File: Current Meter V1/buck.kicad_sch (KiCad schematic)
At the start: 13 parts, among them SW1 SW_DIP_x01, U2 TPS5430DDAR

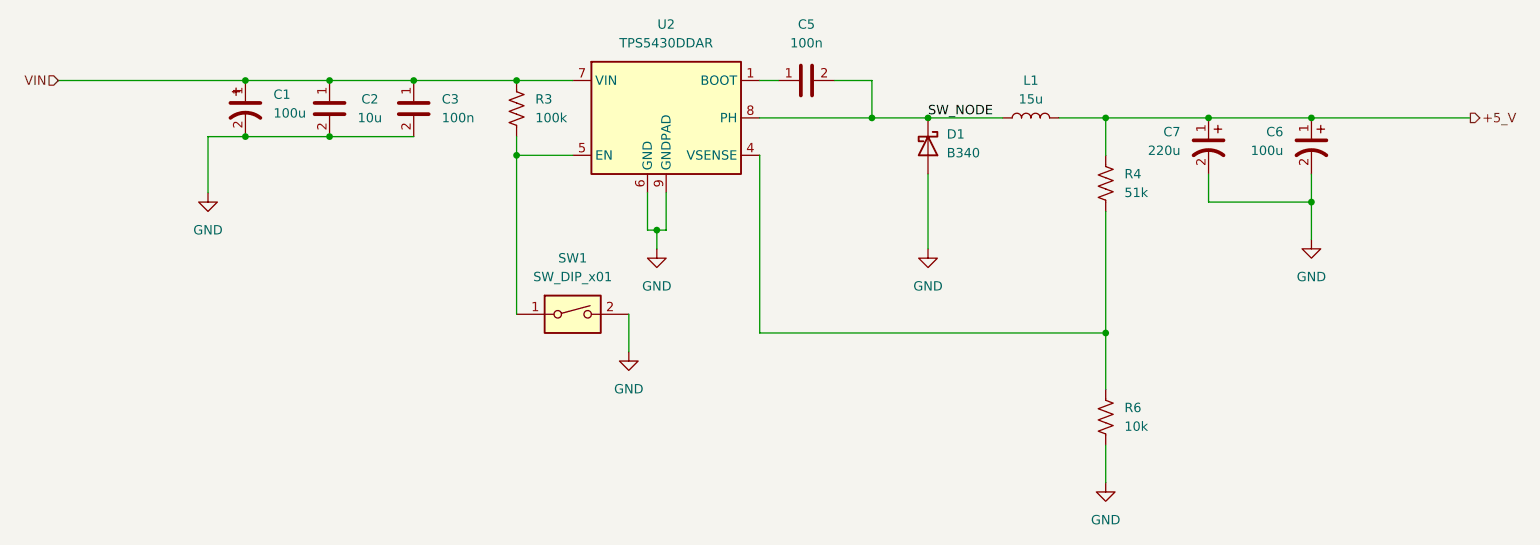
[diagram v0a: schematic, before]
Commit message: buck
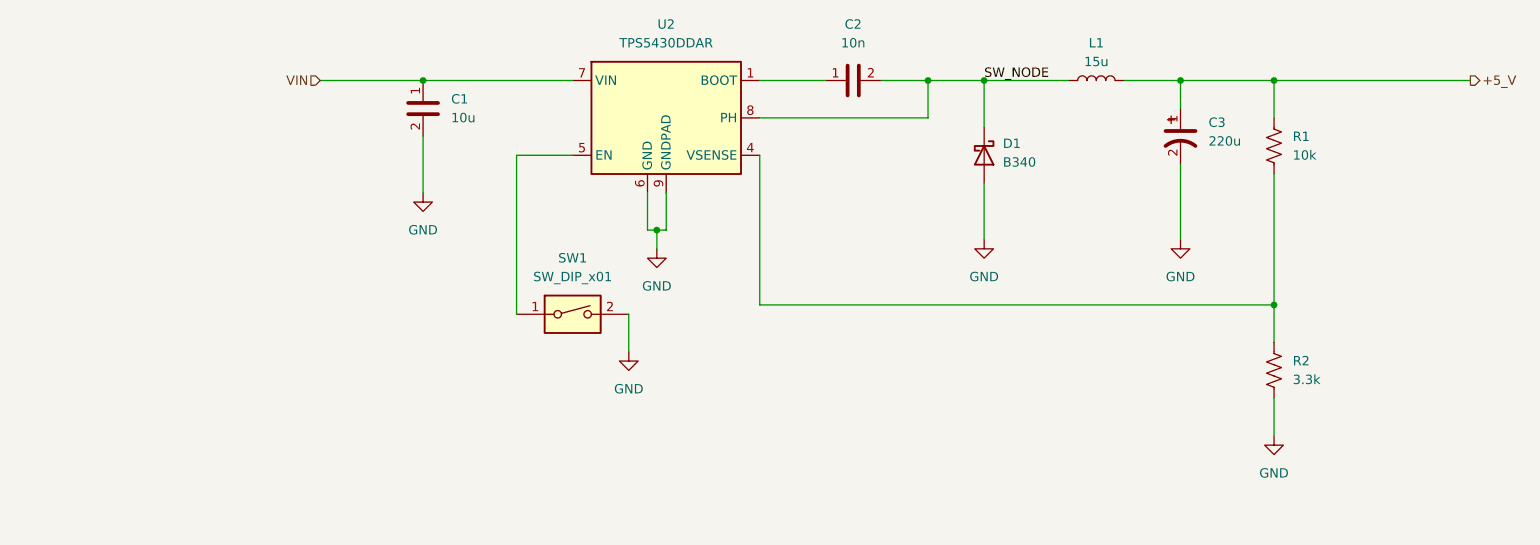
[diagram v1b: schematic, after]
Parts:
- removed C1, C6: 100u, Capacitor_THT:CP_Radial_D8.0mm_P3.50mm, symbol bfr_capacitors:50ZLH100MEFC8X11.5
- removed C2: 10u, Capacitor_SMD:C_0603_1608Metric, symbol bfr_capacitors:CL05A106MQ5NUNC
- removed C3, C5: 100n, Capacitor_SMD:C_0402_1005Metric_Pad0.74x0.62mm_HandSolder, symbol bfr_capacitors:CL05B104KB54PNC
- removed C7: 220u, Capacitor_THT:CP_Radial_D8.0mm_P3.50mm, symbol bfr_capacitors:35ZLH220MEFC8X11.5
- removed R3: 100k, Resistor_SMD:R_0402_1005Metric_Pad0.72x0.64mm_HandSolder, symbol bfr_resistors:RMCF0402FT100K
- removed R4: 51k, Resistor_SMD:R_0402_1005Metric_Pad0.72x0.64mm_HandSolder, symbol bfr_resistors:RMCF0402FT51K0
- removed R6: 10k, Resistor_SMD:R_0402_1005Metric_Pad0.72x0.64mm_HandSolder, symbol bfr_resistors:RMCF0402FT10K0
- added C1: 10u, Capacitor_SMD:C_0603_1608Metric_Pad1.08x0.95mm_HandSolder, symbol bfr_capacitors:CL10A106MA8NRNC
- added C2: 10n, Capacitor_SMD:C_0603_1608Metric_Pad1.08x0.95mm_HandSolder, symbol bfr_capacitors:VJ0603Y103KXAAC
- added C3: 220u, Capacitor_THT:CP_Radial_D8.0mm_P3.50mm, symbol bfr_capacitors:35ZLH220MEFC8X11.5
- added R1: 10k, Resistor_SMD:R_0805_2012Metric_Pad1.20x1.40mm_HandSolder, symbol bfr_resistors:RMCF0805FT10K0
- added R2: 3.3k, Resistor_SMD:R_0805_2012Metric_Pad1.20x1.40mm_HandSolder, symbol bfr_resistors:RMCF0805FT3K30
- L1: footprint Inductor_SMD:L_6.3x6.3_H3 -> bfr_inductors:CDRH104RNP-150NC
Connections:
- net +5_V: now also C3.1, R1.2
- net GND: now also C1.2, C3.2, R2.1
- net SW_NODE: now also C2.2
- net VIN: now also C1.1
- net at U2.4 (VSENSE): now also R1.1, R2.2
- net at U2.1 (BOOT): now also C2.1
